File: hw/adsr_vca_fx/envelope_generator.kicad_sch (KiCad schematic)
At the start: 11 parts, among them J6 Conn_02x05_Odd_Even, SW1 SW_Push, U3 STM32L432KBUx

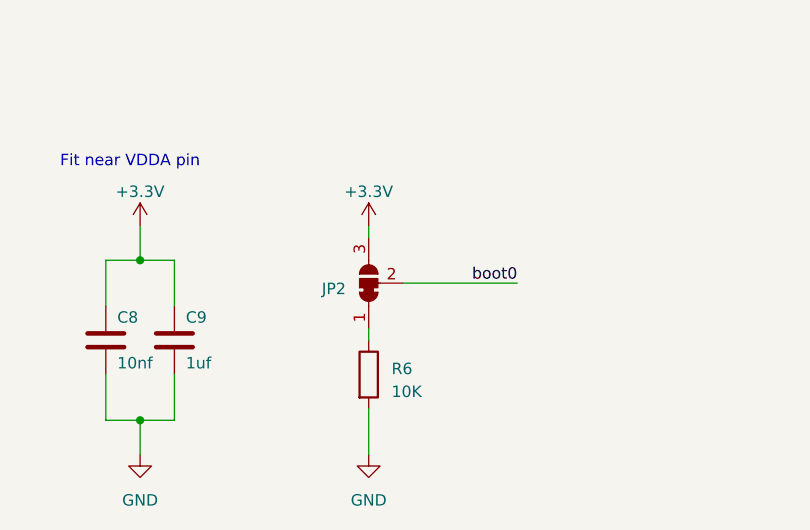
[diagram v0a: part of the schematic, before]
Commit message: tidied up layout
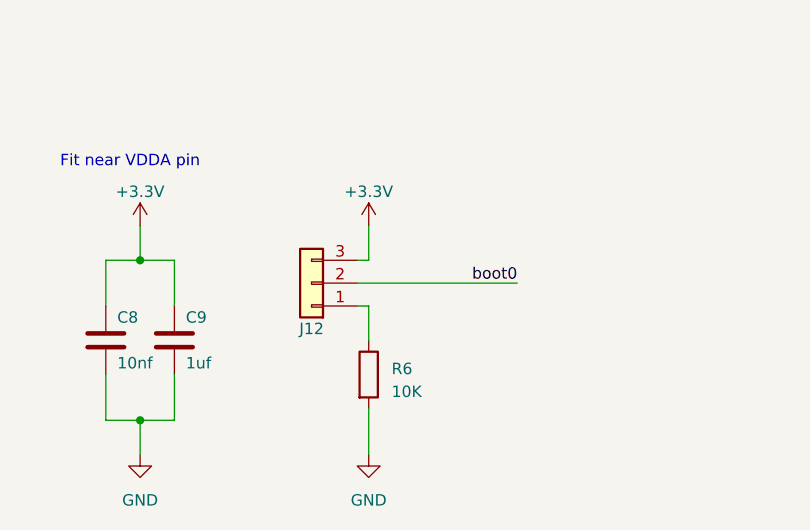
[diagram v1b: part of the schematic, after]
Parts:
- removed JP2: SolderJumper_3_Bridged12, Jumper:SolderJumper-3_P1.3mm_Bridged12_Pad1.0x1.5mm, symbol Jumper:SolderJumper_3_Bridged12
- added J12: Conn_01x03, Connector_PinHeader_2.54mm:PinHeader_1x03_P2.54mm_Vertical, symbol Connector_Generic:Conn_01x03
- JP1: footprint Connector_PinSocket_2.54mm:PinSocket_1x02_P2.54mm_Vertical -> Connector_PinHeader_2.54mm:PinHeader_1x02_P2.54mm_Vertical
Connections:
- net +3.3V: now also J12.3 (Pin_3)
- net boot0: now also J12.2 (Pin_2)
- net at R6.1: now also J12.1 (Pin_1)
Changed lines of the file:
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@@
     (stroke (width 0) (type default))
   )
-  (wire (pts (xy 146.05 162.56) (xy 146.05 163.83))
+  (wire (pts (xy 144.78 154.94) (xy 146.05 154.94))
+    (stroke (width 0) (type default))
+  )
+  (wire (pts (xy 146.05 160.02) (xy 146.05 163.83))
     (stroke (width 0) (type default))
   )
@@
     (stroke (width 0) (type default))
   )
-  (wire (pts (xy 149.86 157.48) (xy 162.56 157.48))
+  (wire (pts (xy 144.78 157.48) (xy 162.56 157.48))
     (stroke (width 0) (type default))
   )
@@
     (stroke (width 0) (type default))
   )
-  (wire (pts (xy 146.05 151.13) (xy 146.05 152.4))
+  (wire (pts (xy 146.05 151.13) (xy 146.05 154.94))
     (stroke (width 0) (type default))
   )
@@
   )
   (bus (pts (xy 245.11 55.88) (xy 245.11 59.69))
+    (stroke (width 0) (type default))
+  )
+  (wire (pts (xy 146.05 160.02) (xy 144.78 160.02))
     (stroke (width 0) (type default))
   )
@@
         (path "/2c7cc946-dcca-4ffb-b6a0-bf0c9ddb491b/1d3f5b6b-6d64-41ce-b32c-1d62b69c11ca"
           (reference "#PWR033") (unit 1)
-        )
-      )
-    )
-  )
-  (symbol (lib_id "Jumper:SolderJumper_3_Bridged12") (at 146.05 157.48 90) (unit 1)
-    (in_bom yes) (on_board yes) (dnp no) (fields_autoplaced)
-    (property "Reference" "JP2" (at 143.51 158.115 90)
-      (effects (font (size 1.27 1.27)) (justify left))
-    )
-    (property "Value" "SolderJumper_3_Bridged12" (at 143.51 159.385 90)
-      (effects (font (size 1.27 1.27)) (justify left) hide)
-    )
-    (property "Footprint" "Jumper:SolderJumper-3_P1.3mm_Bridged12_Pad1.0x1.5mm" (at 146.05 157.48 0)
-      (effects (font (size 1.27 1.27)) hide)
-    )
-    (property "Datasheet" "~" (at 146.05 157.48 0)
-      (effects (font (size 1.27 1.27)) hide)
-    )
-    (pin "1")
-    (pin "2")
-    (pin "3")
-    (instances
-      (project "adsr_vca_fx"
-        (path "/2c7cc946-dcca-4ffb-b6a0-bf0c9ddb491b/1d3f5b6b-6d64-41ce-b32c-1d62b69c11ca"
-          (reference "JP2") (unit 1)
         )
       )
@@
       (effects (font (size 1.27 1.27)))
     )
-    (property "Footprint" "Connector_PinSocket_2.54mm:PinSocket_1x02_P2.54mm_Vertical" (at 64.77 95.25 0)
+    (property "Footprint" "Connector_PinHeader_2.54mm:PinHeader_1x02_P2.54mm_Vertical" (at 64.77 95.25 0)
       (effects (font (size 1.27 1.27)) hide)
     )
@@
         )
       )
+    )
+  )
+  (symbol (lib_id "Connector_Generic:Conn_01x03") (at 139.7 157.48 180) (unit 1)
+    (in_bom yes) (on_board yes) (dnp no)
+    (property "Reference" "J12" (at 139.7 162.56 0)
+      (effects (font (size 1.27 1.27)))
+    )
+    (property "Value" "Conn_01x03" (at 139.7 162.56 0)
+      (effects (font (size 1.27 1.27)) hide)
+    )
+    (property "Footprint" "Connector_PinHeader_2.54mm:PinHeader_1x03_P2.54mm_Vertical" (at 139.7 157.48 0)
+      (effects (font (size 1.27 1.27)) hide)
+    )
+    (property "Datasheet" "~" (at 139.7 157.48 0)
+      (effects (font (size 1.27 1.27)) hide)
+    )
+    (pin "1")
+    (pin "2")
+    (pin "3")
+    (instances
+      (project "adsr_vca_fx"
+        (path "/2c7cc946-dcca-4ffb-b6a0-bf0c9ddb491b/1d3f5b6b-6d64-41ce-b32c-1d62b69c11ca"
+          (reference "J12") (unit 1)
+        )
+      )
